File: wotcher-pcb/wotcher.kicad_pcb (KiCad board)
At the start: 2 copper layers, 40.1 x 39.6 mm, 105 parts, among them CN1 SM02B-SRSS-TB, SW1 SKTDLHE010, SW2 SKTDLHE010, SW3 SKTDLHE010, SW4 SKTDLHE010, U1 KCSA02-105, U2 KCSA02-105, U3 LIS2DW12TR-MS, U5 ATtiny1616-M, U6 KCSA02-105, U7 IS31FL3731-QF, U8 KCSA02-105, U9 DS3231MZ+

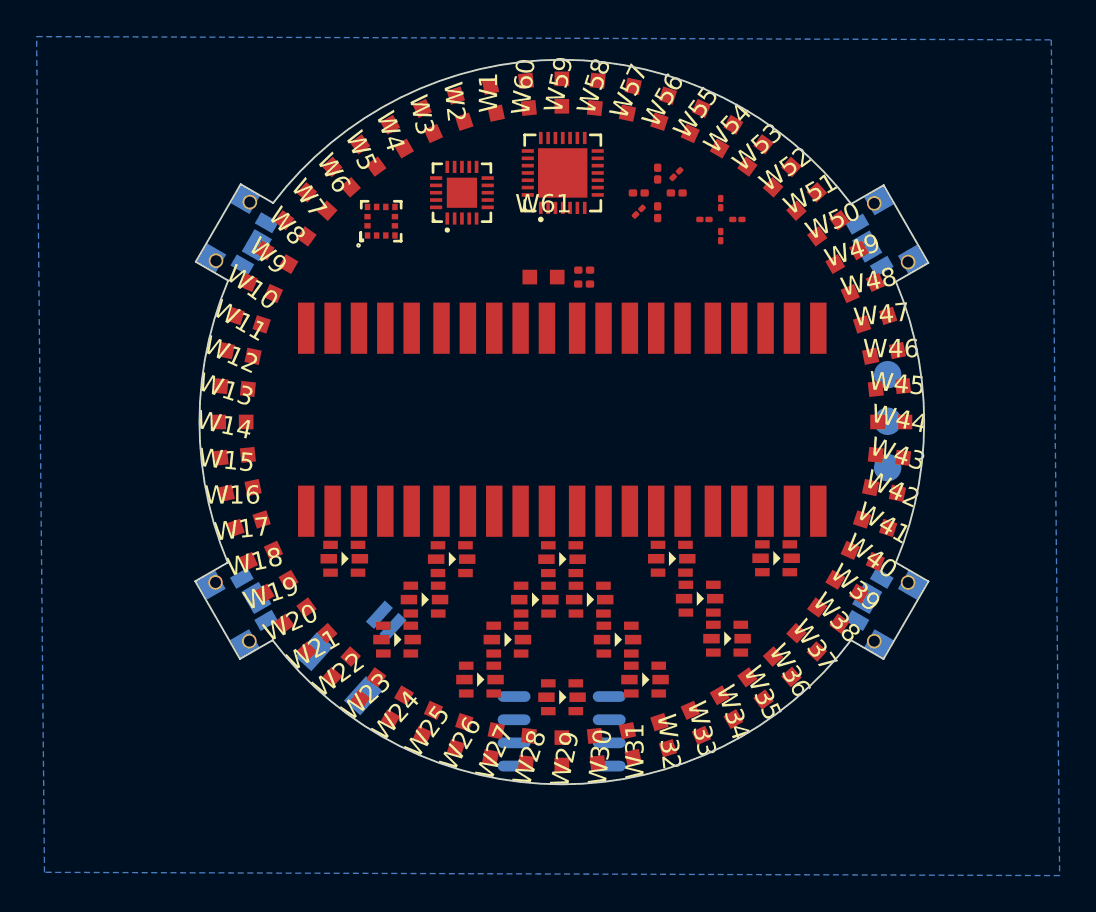
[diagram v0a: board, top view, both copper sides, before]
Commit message: add step file
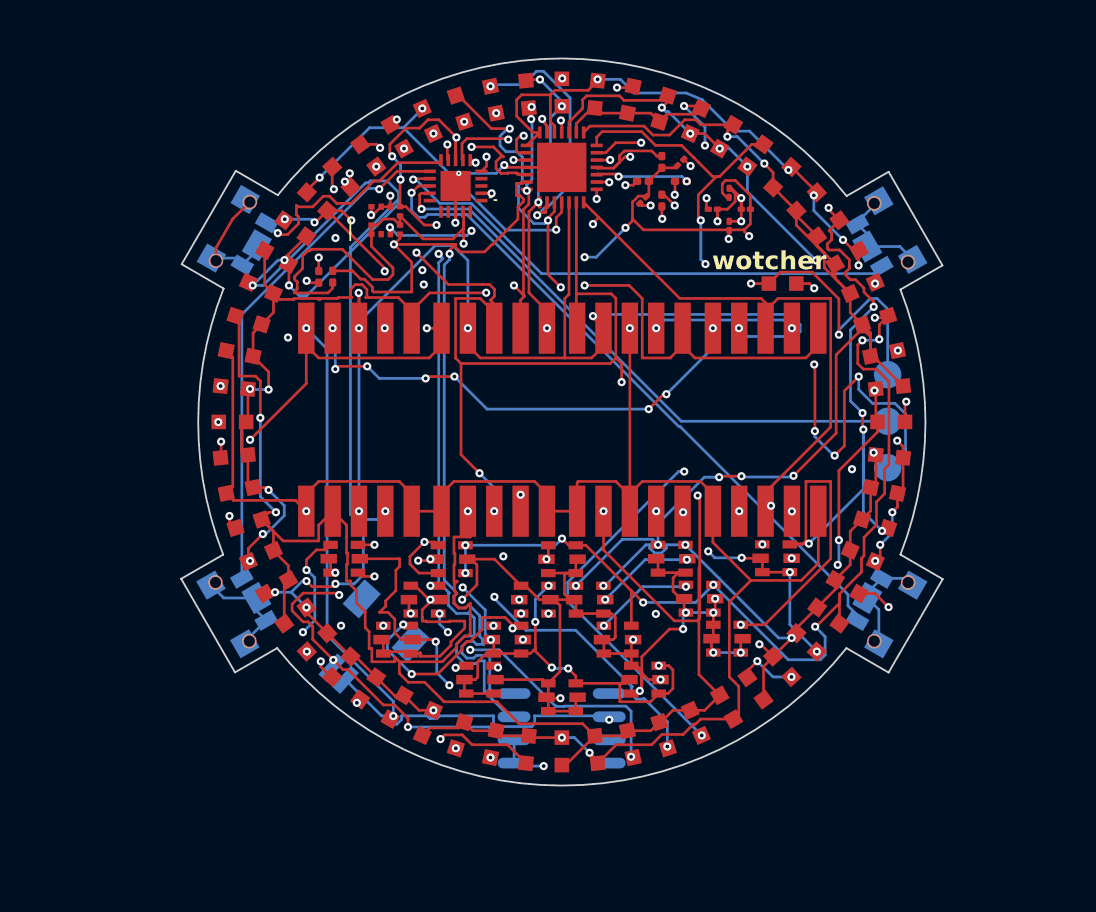
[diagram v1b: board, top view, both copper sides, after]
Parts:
- moved R6 14.5 mm to (51.7, 37.1), turned to -90 degrees
- moved R2 13.7 mm to (52.5, 37.1), turned to 90 degrees
- moved W61 13.1 mm to (77.1, 37.4)
- moved C1 0.72 mm to (74.1, 32.5)
- moved C2 0.72 mm to (75.1, 33.4)
- moved C3 0.72 mm to (73.3, 33.4)
- moved C4 0.72 mm to (74.1, 34.3)
- moved C6 0.67 mm to (69.4, 32.9)
- moved R5 0.67 mm to (70.5, 32.9)
- moved C5 0.67 mm to (71.5, 30.8)
- moved R3 0.67 mm to (69.4, 31.9)
- moved R4 0.67 mm to (71.5, 31.9)
- moved R1 0.67 mm to (70.5, 30.8)
- moved U5 0.50 mm to (59.2, 32.1)
- moved U7 0.31 mm to (65.0, 31.1), turned to 90 degrees
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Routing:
- net CB6: track 0.00 -> 177.3 mm, vias 0 -> 23
- net CA7: track 0.00 -> 137.6 mm, vias 0 -> 18
- net CA4: track 0.00 -> 136.7 mm, vias 0 -> 9
- net ATtinyVCC: track 0.00 -> 133.4 mm, vias 0 -> 10
- net CA3: track 0.00 -> 127.5 mm, vias 0 -> 15
- net CA5: track 0.00 -> 127.5 mm, vias 0 -> 9
- net CA8: track 0.00 -> 121.2 mm, vias 0 -> 11
- net CA6: track 0.00 -> 116.1 mm, vias 0 -> 12
- net CB1: track 0.00 -> 110.5 mm, vias 0 -> 13
- net CB7: track 0.00 -> 101.4 mm, vias 0 -> 16
- net CB5: track 0.00 -> 99.6 mm, vias 0 -> 15
- net CB2: track 0.00 -> 97.6 mm, vias 0 -> 14
- net CB4: track 0.00 -> 95.9 mm, vias 0 -> 20
- net CA1: track 0.00 -> 94.6 mm, vias 0 -> 21
- net CA2: track 0.00 -> 93.0 mm, vias 0 -> 12
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- added copper zone on In1.Cu, net ATtinyGND
- removed copper zone on B.Cu, net ATtinyGND
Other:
- board size 40.1 x 39.6 mm -> 41.6 x 39.7 mm
- copper layers 2 -> 4
- board text added: "wotcher"
